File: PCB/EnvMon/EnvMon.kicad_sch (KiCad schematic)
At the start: 40 parts, among them J1 USB-C, J2 DC, J3 TEMP, J4 Shelly, M1 OLED1.5-RGB, SW1 SW_Push, SW2 SW_Push, SW3 SW_Push, U1 LMR16006XDDCR, U2 SCD41, U3 FT231XQ, U4 ESP32-PICO-MINI-02, U5 QR, U7 SHT40, U8 VEML6040

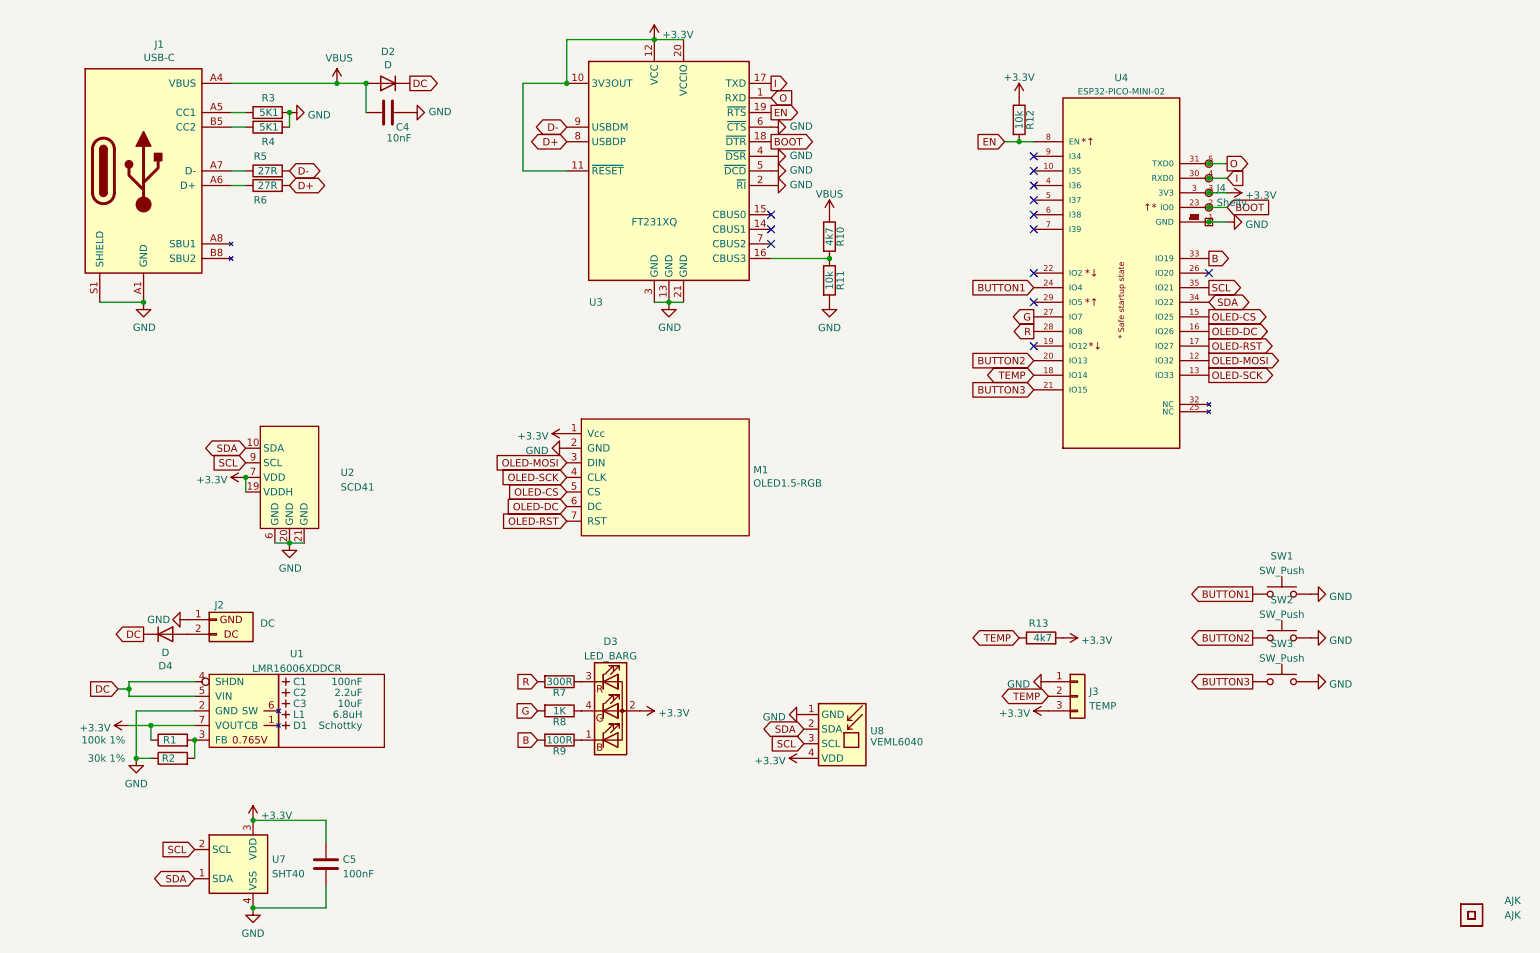
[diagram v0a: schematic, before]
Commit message: One board
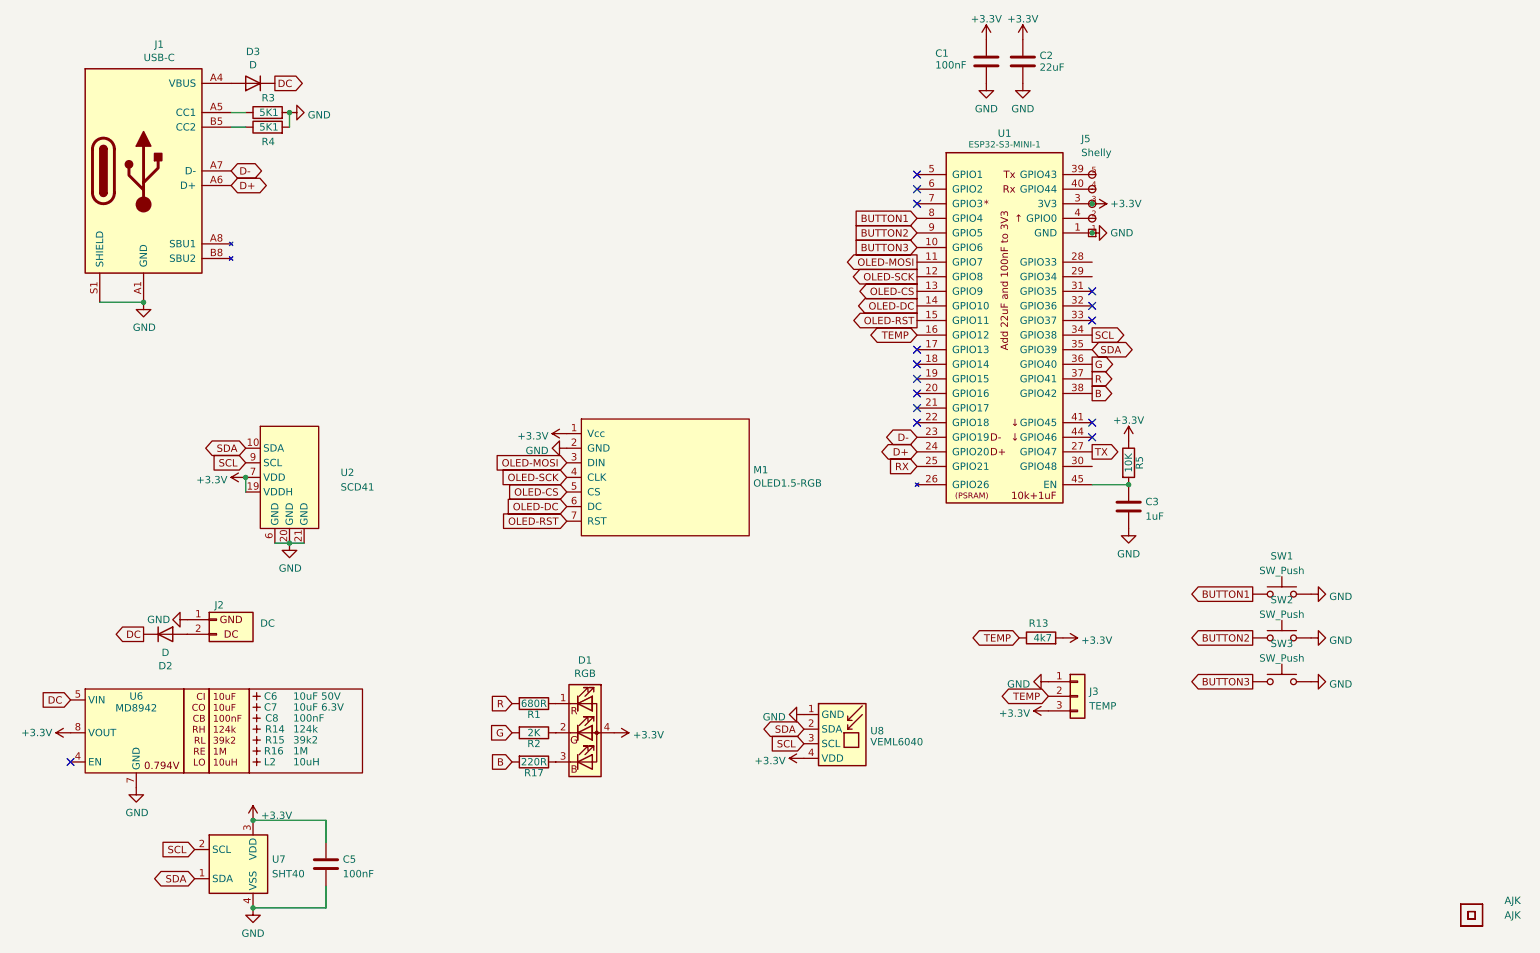
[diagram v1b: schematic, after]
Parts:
- removed C1: 100nF, RevK:C_0603_, symbol RevK:Hidden
- removed C2: 2.2uF, RevK:C_0805_, symbol RevK:Hidden
- removed C3: 10uF, RevK:C_0805_, symbol RevK:Hidden
- removed C4: 10nF, RevK:C_0603, symbol Device:C
- removed D1: Schottky, RevK:D_1206_, symbol RevK:Hidden
- removed D3: LED_BARG, RevK:MHS190RGBCT, symbol Device:LED_BARG
- removed D4: D, RevK:D_1206, symbol Device:D
- removed J4: Shelly, RevK:Shelly, symbol RevK:Shelly
- removed L1: 6.8uH, RevK:L_4x4_, symbol RevK:Hidden
- removed R10: 4k7, RevK:R_0603, symbol Device:R
- removed R11, R12: 10k, RevK:R_0603, symbol Device:R
- removed R6: 27R, RevK:R_0603, symbol Device:R
- removed R7: 300R, RevK:R_0603, symbol Device:R
- removed R8: 1K, RevK:R_0603, symbol Device:R
- removed R9: 100R, RevK:R_0603, symbol Device:R
- removed U1: LMR16006XDDCR, RevK:SOT-23-Thin-6-Reg, symbol RevK:LMR16006XDDCR
- removed U3: FT231XQ, RevK:QFN-20-1EP_4x4mm_P0.5mm_EP2.5x2.5mm, symbol RevK:FT231XQ
- removed U4: ESP32-PICO-MINI-02, RevK:ESP32-PICO-MINI-02, symbol RevK:ESP32-PICO-MINI-02
- added C1: 100nF, RevK:C_0402, symbol Device:C
- added C2: 22uF, RevK:C_0402, symbol Device:C
- added C3: 1uF, RevK:C_0402, symbol Device:C
- added C6: 10uF 50V, RevK:C_0603_, symbol RevK:Hidden
- added C7: 10uF 6.3V, RevK:C_0603_, symbol RevK:Hidden
- added C8: 100nF, RevK:C_0603_, symbol RevK:Hidden
- added D1: RGB, RevK:LED-RGB-1.6x1.6, symbol Device:LED_RGBA
- added D3: D, RevK:D_SOD-123, symbol Device:D
- added J5: Shelly, RevK:Shelly, symbol RevK:Shelly
- added L2: 10uH, RevK:L_4x4_, symbol RevK:Hidden
- added R14: 124k, RevK:R_0402_, symbol RevK:Hidden
- added R15: 39k2, RevK:R_0402_, symbol RevK:Hidden
- added R16: 1M, RevK:R_0402_, symbol RevK:Hidden
- added R17: 220R, RevK:R_0402, symbol Device:R
- added U1: ESP32-S3-MINI-1, RevK:ESP32-S3-MINI-1, symbol RevK:ESP32-S3-MINI-1-N4R2
- added U6: MD8942, RevK:SOT-23-6-MD8942, symbol RevK:MD89420-RegBlock
- C5: footprint RevK:C_0603 -> RevK:C_0402
- D2: footprint RevK:D_1206 -> RevK:D_SOD-123; LCSC Part # C143805 -> C1884542
- R1: value 100k 1% -> 680R; footprint RevK:R_0603 -> RevK:R_0402; LCSC Part # C14675 -> (none)
- R13, R3, R4: footprint RevK:R_0603 -> RevK:R_0402
- R2: value 30k 1% -> 2K; footprint RevK:R_0603 -> RevK:R_0402; LCSC Part # C100001 -> (none)
- R5: value 27R -> 10K; footprint RevK:R_0603 -> RevK:R_0402
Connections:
- net +3.3V: now also R5.1, C1.1, C2.1, D1.4 (A), J5.3 (3V3), U1.3 (3V3), U6.8 (VOUT); no longer R1.1
- net B: now also R17.2, U1.38 (GPIO42)
- net BUTTON1: now also U1.8 (GPIO4)
- net BUTTON2: now also U1.9 (GPIO5)
- net BUTTON3: now also U1.10 (GPIO6)
- net D+: now also J1.A6 (D+), J1.B6 (D+), U1.24 (GPIO20)
- net D-: now also J1.A7 (D-), J1.B7 (D-), U1.23 (GPIO19); no longer R5.2
- net DC: now also D3.1 (K), U6.5 (VIN)
- net G: now also R2.2, U1.36 (GPIO40)
- net GND: now also C1.2, C2.2, C3.2, J5.1 (GND), U1.1 (GND), U1.2 (GND), U1.42 (GND), U1.43 (GND), U1.46 (GND), U1.47 (GND), U1.48 (GND), U1.49 (GND), U1.50 (GND), U1.51 (GND), U1.52 (GND), U1.53 (GND), U1.54 (GND), U1.55 (GND), U1.56 (GND), U1.57 (GND), U1.58 (GND), U1.59 (GND), U1.60 (GND), U1.61 (GND), U1.62 (GND), U1.63 (GND), U1.64 (GND), U1.65 (GND), U6.2 (GND), U6.7 (GND); no longer R2.1
- net OLED-CS: now also U1.13 (GPIO9)
- net OLED-DC: now also U1.14 (GPIO10)
- net OLED-MOSI: now also U1.11 (GPIO7)
- net OLED-RST: now also U1.15 (GPIO11)
- net OLED-SCK: now also U1.12 (GPIO8)
- net R: now also R1.2, U1.37 (GPIO41)
- net SCL: now also U1.34 (GPIO38)
- net SDA: now also U1.35 (GPIO39)
- net TEMP: now also U1.16 (GPIO12)
- net at J2.2 (DC): now also D2.2 (A)
- net VBUS: no longer names the net of J1.A4 (VBUS), J1.A9 (VBUS), J1.B4 (VBUS), J1.B9 (VBUS)
- net VBUS: now also D3.2 (A); no longer D2.2 (A)
- new net: J5.2 (0), U1.4 (GPIO0)
- new net: J5.4 (Rx), U1.40 (GPIO44)
- new net: J5.5 (Tx), U1.39 (GPIO43)
- new net: D1.2 (GK), R2.1
- new net: C3.1, R5.2, U1.45 (EN)
- new net: D1.1 (RK), R1.1
- new net: D1.3 (BK), R17.1
- new net RX: U1.25 (GPIO21)
- new net TX: U1.27 (GPIO47)
- no-connect marks 13 -> 15
